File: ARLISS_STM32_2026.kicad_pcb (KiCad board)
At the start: 4 copper layers, 118 parts, among them CN1 XT30PW-M, CN2 XT30PW-M, CN3 DB127V-5.08-2P-GN-S, CN4 0430450400, J1 Conn_01x06, J2 Conn_01x06, P1 PZ254R-12-8P, Q1 IRLZ44NPBF, Q2 AOD4185_C400894, Q3 AOD4185_C400894, SW1 EVQPLMA15, SW2 EVQPLMA15, U1 STM32F405RGT6, U10 INA226AIDGSR, U11 INA226AIDGSR, U12 ADXL375BCCZ, U2 4754, U3 DRV8874PWPR, U4 DRV8874PWPR, U5 BMP581, U6 VEML7700-TR, U7 AP63203QWU-7, X1 32.768kHz 7pF SMD, X2 8Mhz 10pF

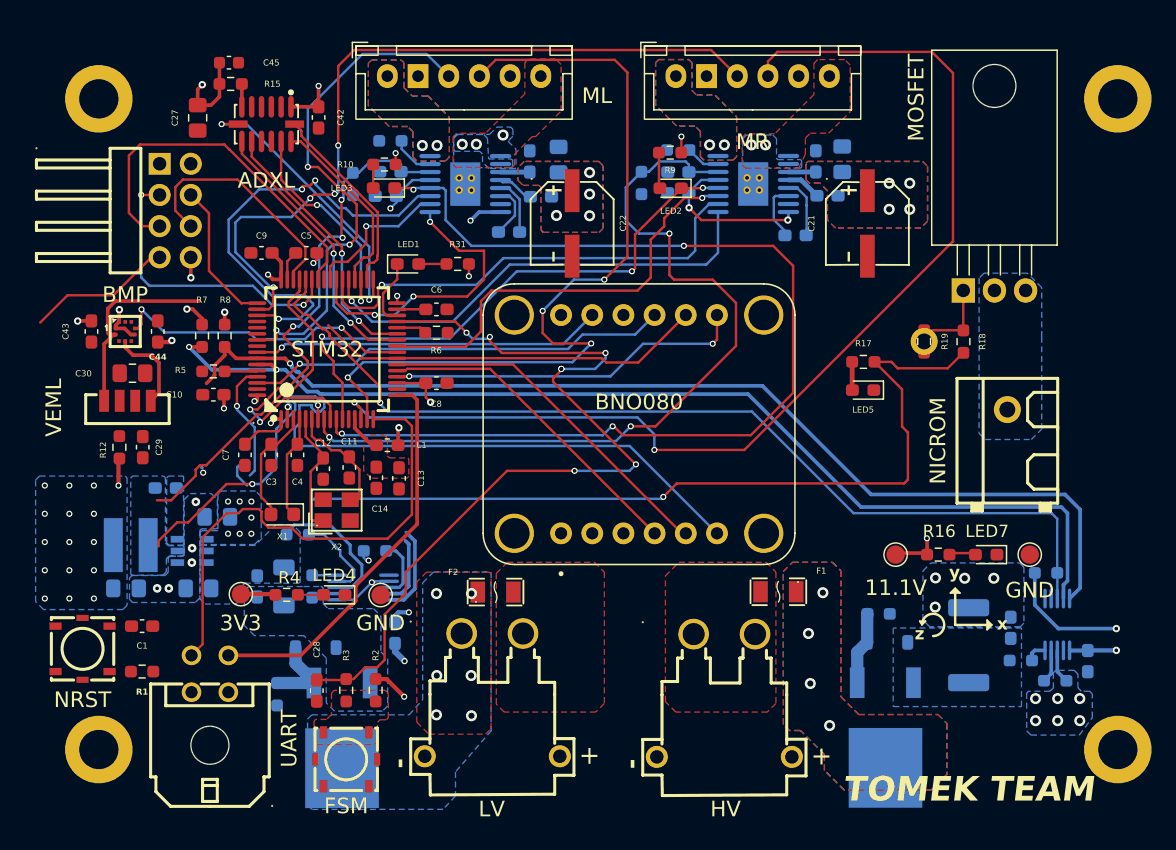
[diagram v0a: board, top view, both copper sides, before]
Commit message: FINAL
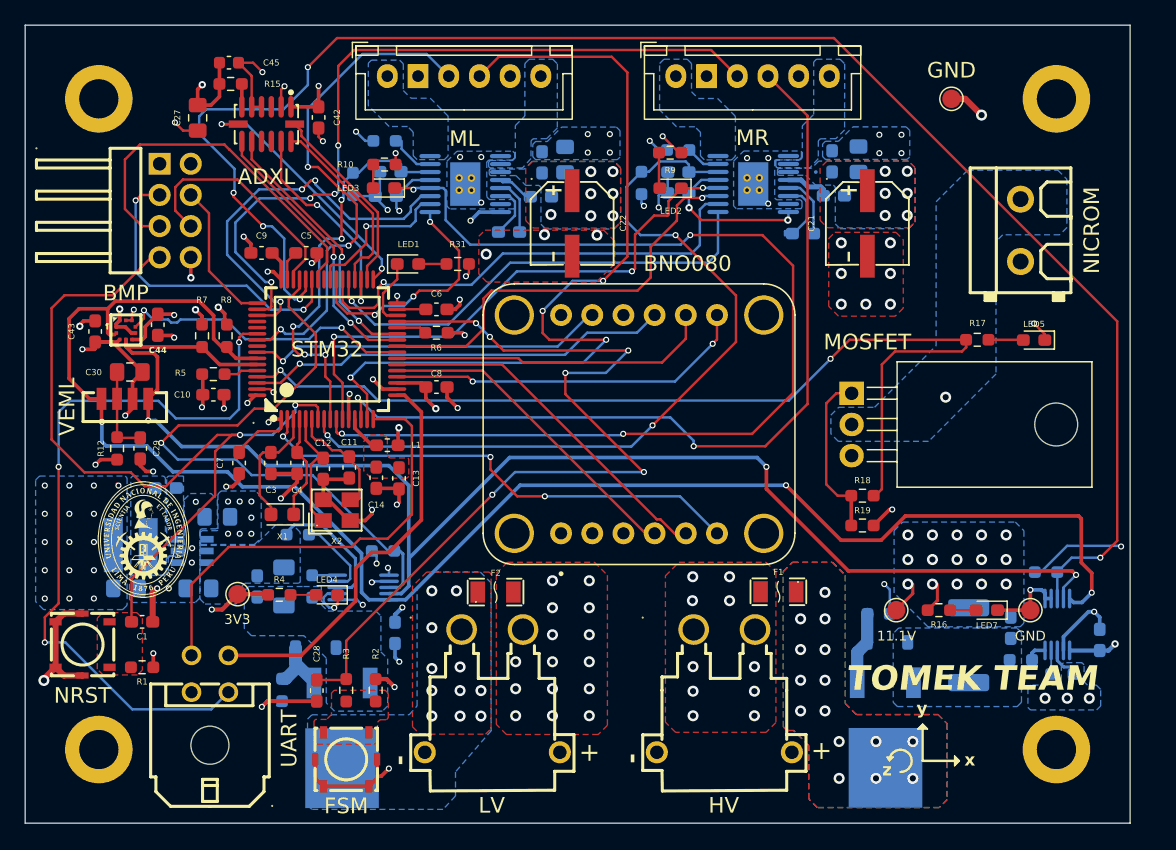
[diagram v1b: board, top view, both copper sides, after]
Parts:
- added G***: LOGO, LOGO, F.Cu at (67.5, 110.3)
- added G***: LOGO, LOGO, B.Cu at (107.9, 100.8)
- moved TP4 61.6 mm to (133.3, 74.4)
- moved CN3 17.2 mm to (139.0, 85.1)
- moved R19 15.8 mm to (126.1, 109.2), turned to 180 degrees
- moved R18 15.0 mm to (126.1, 106.7), turned to 180 degrees
- moved LED5 14.5 mm to (140.1, 94.0)
- moved Q1 12.4 mm to (125.2, 98.4), turned to -90 degrees
- moved R17 9.45 mm to (135.4, 94.0), turned to 0 degrees
- moved H4 5.00 mm to (141.9, 74.4)
- moved H5 5.00 mm to (141.9, 127.4)
- moved LED7 4.53 mm to (136.2, 116.0)
- moved R16 4.53 mm to (132.3, 116.0)
- moved TP2 4.53 mm to (128.8, 116.0)
- moved TP3 4.53 mm to (139.8, 116.0)
- moved C39 1.98 mm to (145.4, 118.5), turned to -90 degrees
- moved C23 1.33 mm to (123.6, 79.5)
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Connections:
- U1 pad 54: unconnected-(U1A-PD2-Pad54) -> /CORE_STM32F405/RADXA_PIN
- U3 pad : (no net) -> GND
- U4 pad : (no net) -> GND
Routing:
- net GND: track 2.70 -> 139.8 mm, vias 7 -> 68
- net /CORE_STM32F405/RADXA_PIN: track 0.00 -> 60.6 mm, vias 0 -> 3
- net ALERT1_INA226: track 79.3 -> 134.7 mm, vias 1 -> 5
- net /CORE_STM32F405/NRST: track 34.0 -> 68.2 mm, vias 3 -> 2
- net I2C1_SCL: track 110.0 -> 135.7 mm, vias 1 -> 3
- net ENCODER_B_1: track 90.7 -> 69.8 mm
- net I2C1_SDA: track 99.9 -> 120.7 mm, vias 2 -> 3
- net ALERT2_INA226: track 30.9 -> 50.7 mm, vias 0 -> 1
- net ADC2: track 43.0 -> 33.0 mm
- net IMU INT: track 49.1 -> 40.8 mm, vias 1 -> 3
- net /Heating_resistance/Mosfet_G: track 5.99 -> 13.9 mm
- net /VEML 7700 Sheet/VDD_LUZ: track 0.00 -> 7.42 mm
- net SPI1_MOSI: track 32.0 -> 26.4 mm
- net nSLEEP2: track 36.4 -> 31.8 mm
- net /CORE_STM32F405/TX2: track 40.8 -> 36.7 mm
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- added copper zone on In2.Cu, net +3.3V
- added copper zone on F.Cu, net /CORE_STM32F405/NRST
- added copper zone on F.Cu, net GND
- added copper zone on In1.Cu, net GND
- removed copper zone on F.Cu, net /Motor control/M1+
- removed copper zone on F.Cu, net /Motor control/M1-
- removed copper zone on F.Cu, net /Motor control/M2+
- removed copper zone on F.Cu, net /Motor control/M2-
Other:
- board outline added: 90 x 65 mm
- board text added: "Carlos Yujra"
- board text added: "Jair Oria"
- board text added: "Jhamir Mamani"
- board text added: "MEMBERS:"
- board text added: "Osmer Diaz"
- board text added: "Pedro Palacios"
